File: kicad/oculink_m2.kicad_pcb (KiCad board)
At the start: 4 copper layers, 100.5 x 112.3 mm, 17 parts, among them J1 G14A421211112HR

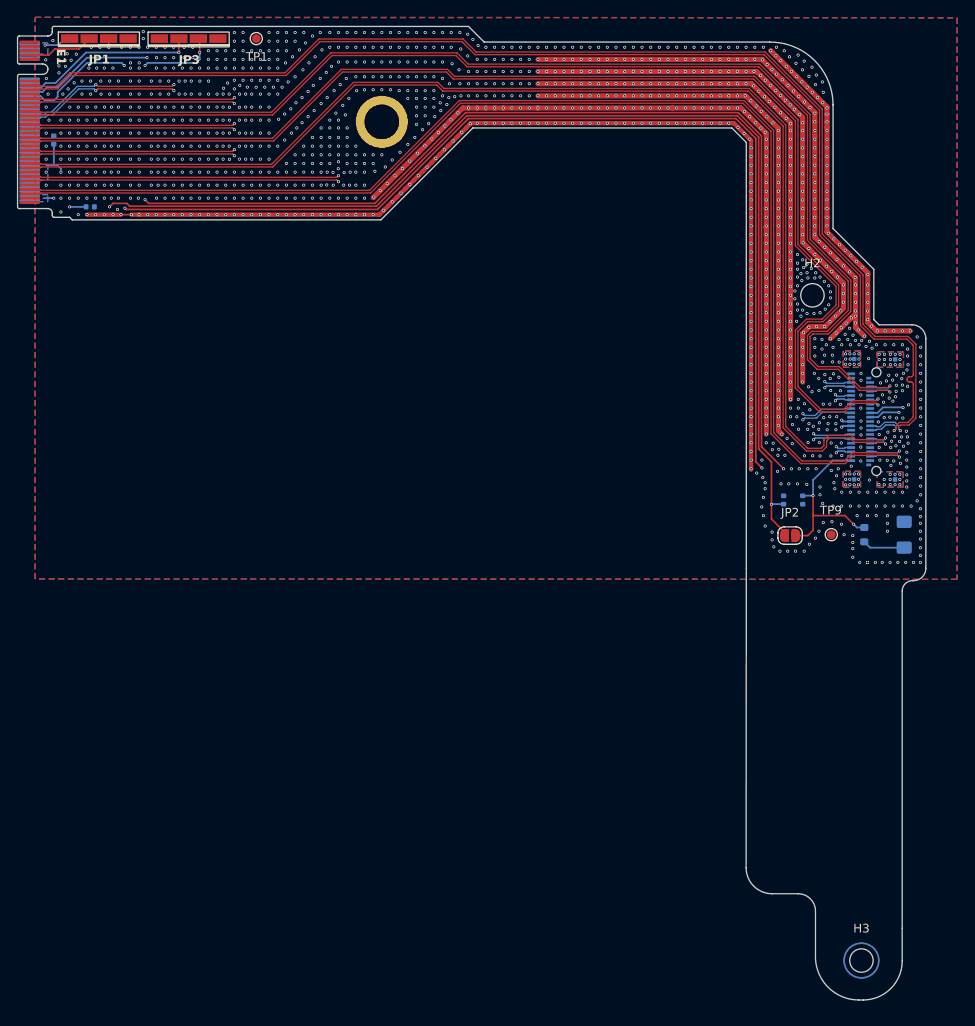
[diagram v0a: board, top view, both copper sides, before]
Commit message: Fixed position of additional mounting holes and made them oval vertically for potential vertical adjustment of adapter
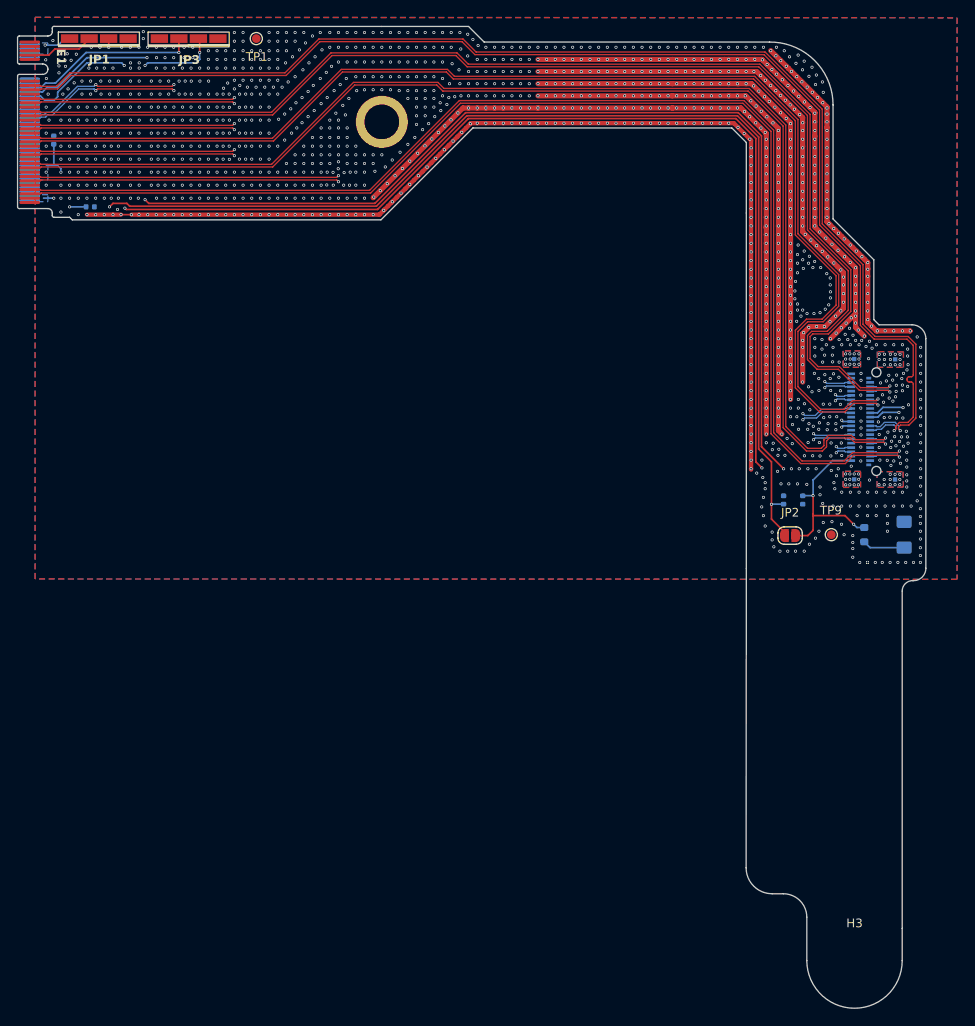
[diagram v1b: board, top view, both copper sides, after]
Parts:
- moved H3 1.00 mm to (187.5, 147.1)
- moved H2 0.65 mm to (182.7, 70.3)
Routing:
- net GND: track 965.6 -> 965.8 mm, vias 1493 -> 1492
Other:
- board size 100.5 x 112.3 mm -> 100.5 x 113.2 mm

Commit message: Fixed ground pour overflowing onto m2 edge connector
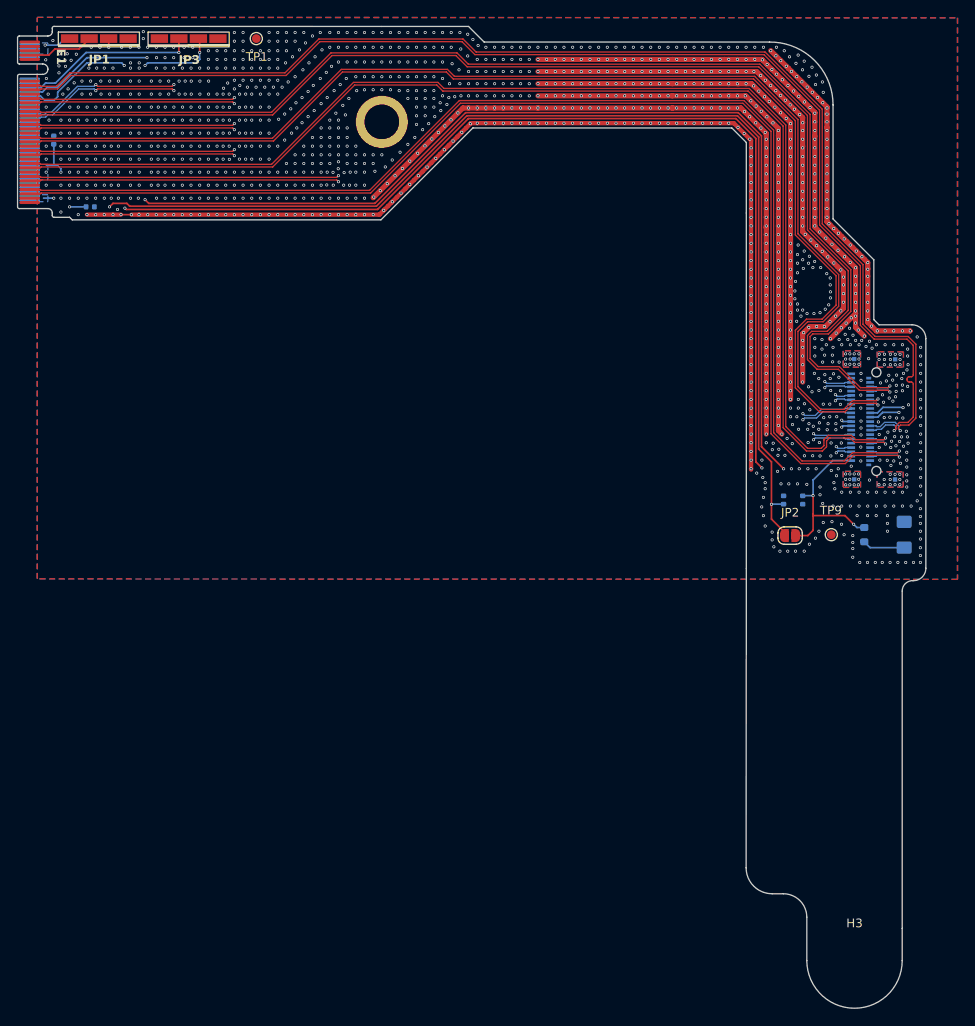
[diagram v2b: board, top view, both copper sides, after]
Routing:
- net GND: vias 1492 -> 1491
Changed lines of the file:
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@@
 	)
 	(via
-		(at 189 101.8)
-		(size 0.35)
-		(drill 0.2)
-		(layers "F.Cu" "B.Cu")
-		(free yes)
-		(net 1)
-	)
-	(via
 		(at 126 52.8)
 		(size 0.35)
@@
 		(polygon
 			(pts
-				(xy 93.025 38.95) (xy 199.325 39) (xy 199.325 103.75) (xy 93.025 103.7)
+				(xy 93.275 38.95) (xy 199.375 39) (xy 199.375 103.75) (xy 93.275 103.7)
 			)
 		)

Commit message: Added stackup information to schematic
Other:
- board text added: "0"
- board text added: "0 mm"
- board text added: "0.0152 mm"
- board text added: "0.01524 mm"
- board text added: "0.02"
- board text added: "0.035 mm"
- board text added: "0.0900 mm / 0.0900 mm"
- board text added: "0.0994 mm"
- board text added: "0.1500 mm"
- board text added: "0.45 mm"
- board text added: "0.7797 mm"
- board text added: "1"
- board text added: "104.7250 mm x 113.2111 mm"
- board text added: "3.8"
- board text added: "3113x1"
- board text added: "4"
- board text added: "4.1"
- board text added: "4.6"
- board text added: "B.Cu"
- board text added: "B.Mask"
- board text added: "B.Paste"
- board text added: "B.Silkscreen"
- board text added: "BOARD CHARACTERISTICS"
- board text added: "Board Thickness:"
- board text added: "Board overall dimensions:"
- board text added: "Bottom Silk Screen"
- board text added: "Bottom Solder Mask"
- board text added: "Bottom Solder Paste"
- board text added: "Castellated pads:"
- board text added: "Color"
- board text added: "Copper Finish:"
- board text added: "Copper Layer Count:"
- board text added: "Core"
- board text added: "Dielectric 1"
- board text added: "Dielectric 2"
- board text added: "Dielectric 3"
- board text added: "Direct Printing"
- board text added: "Edge card connectors:"
- board text added: "Epsilon R"
- board text added: "F.Cu"
- board text added: "F.Mask"
- board text added: "F.Paste"
- board text added: "F.Silkscreen"
- board text added: "FR4 natural"
- board text added: "Green"
- board text added: "Impedance Control:"
- board text added: "In1.Cu"
- board text added: "In2.Cu"
- board text added: "Layer Name"
- board text added: "Loss Tangent"
- board text added: "Material"
- board text added: "Min hole diameter:"
- board text added: "Min track/spacing:"
- board text added: "No"
- board text added: "None"
- board text added: "Not specified"
- board text added: "PCIE 4.0 x 4 M2 to Oculink Adapter for 16ARP8 Laptop"
- board text added: "Plated Board Edge:"
- board text added: "Thickness (mm)"
- board text added: "Top Silk Screen"
- board text added: "Top Solder Mask"
- board text added: "Top Solder Paste"
- board text added: "Type"
- board text added: "White"
- board text added: "Yes"
- board text added: "copper"
- board text added: "core"
- board text added: "prepreg"
